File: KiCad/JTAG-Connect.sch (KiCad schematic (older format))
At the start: 2 parts, among them J1 Conn_02x05_Odd_Even, J2 Conn_02x03_Odd_Even

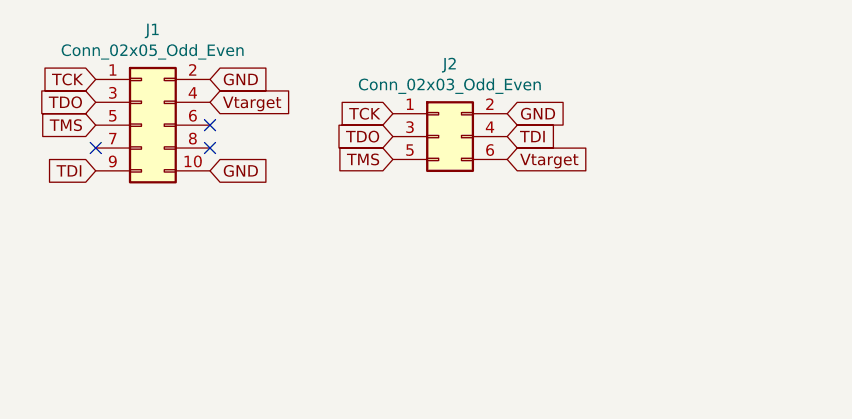
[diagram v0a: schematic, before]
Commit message: updated design
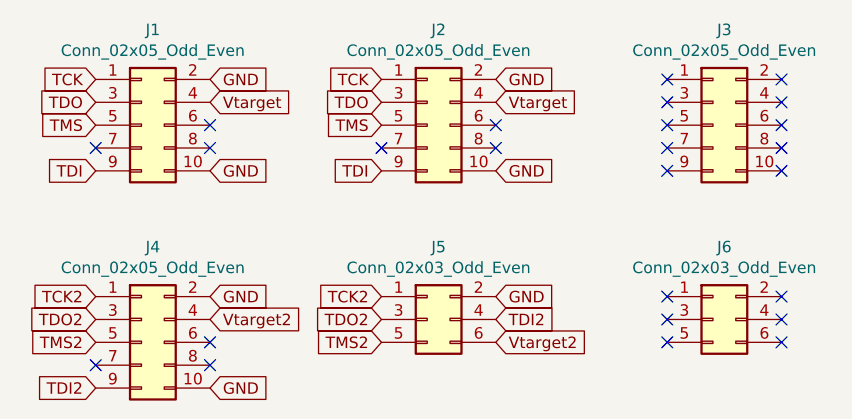
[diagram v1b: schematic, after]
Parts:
- removed J2: Conn_02x03_Odd_Even, Connector_PinHeader_2.00mm:PinHeader_2x03_P2.00mm_Vertical, symbol Connector_Generic:Conn_02x03_Odd_Even
- added J2, J3: Conn_02x05_Odd_Even, JTAG-Connect:PinHeader_2x05_P2.00mm_JTAG_connect_on_SMD_pads, symbol Connector_Generic:Conn_02x05_Odd_Even
- added J4: Conn_02x05_Odd_Even, Connector_IDC:IDC-Header_2x05_P2.54mm_Vertical, symbol Connector_Generic:Conn_02x05_Odd_Even
- added J5, J6: Conn_02x03_Odd_Even, JTAG-Connect:PinHeader_2x03_P2.00mm_JTAG_connect_on_SMD_pads, symbol Connector_Generic:Conn_02x03_Odd_Even
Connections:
- net GND: now also J2.10 (Pin_10), J2.2 (Pin_2), J4.10 (Pin_10), J4.2 (Pin_2), J5.2 (Pin_2)
- net TCK: now also J2.1 (Pin_1)
- net TDI: now also J2.9 (Pin_9)
- net TDO: now also J2.3 (Pin_3)
- net TMS: now also J2.5 (Pin_5)
- net Vtarget: now also J2.4 (Pin_4)
- new net TCK2: J4.1 (Pin_1), J5.1 (Pin_1)
- new net TDI2: J4.9 (Pin_9), J5.4 (Pin_4)
- new net TDO2: J4.3 (Pin_3), J5.3 (Pin_3)
- new net TMS2: J4.5 (Pin_5), J5.5 (Pin_5)
- new net Vtarget2: J4.4 (Pin_4), J5.6 (Pin_6)
- no-connect marks 3 -> 25
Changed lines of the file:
@@
 $EndDescr
-$Comp
-L Connector_Generic:Conn_02x03_Odd_Even J2
-U 1 1 6687D8BE
-P 3650 2650
-F 0 "J2" H 3700 2967 50  0000 C CNN
-F 1 "Conn_02x03_Odd_Even" H 3700 2876 50  0000 C CNN
-F 2 "Connector_PinHeader_2.00mm:PinHeader_2x03_P2.00mm_Vertical" H 3650 2650 50  0001 C CNN
-F 3 "~" H 3650 2650 50  0001 C CNN
-	1    3650 2650
-	1    0    0    -1
-$EndComp
-Text GLabel 3450 2550 0    50   Input ~ 0
-TCK
-Text GLabel 3450 2650 0    50   Input ~ 0
-TDO
-Text GLabel 3450 2750 0    50   Input ~ 0
-TMS
-Text GLabel 3950 2550 2    50   Input ~ 0
-GND
-Text GLabel 3950 2650 2    50   Input ~ 0
-TDI
-Text GLabel 3950 2750 2    50   Input ~ 0
-Vtarget
 $Comp
 L Connector_Generic:Conn_02x05_Odd_Even J1
@@
 TDI
 NoConn ~ 2150 2700
-Text GLabel 2650 2400 2    50   Input ~ 0
+NoConn ~ 2650 2600
+NoConn ~ 2650 2700
+$Comp
+L Connector_Generic:Conn_02x05_Odd_Even J2
+U 1 1 66A23D81
+P 3600 2600
+F 0 "J2" H 3650 3017 50  0000 C CNN
+F 1 "Conn_02x05_Odd_Even" H 3650 2926 50  0000 C CNN
+F 2 "JTAG-Connect:PinHeader_2x05_P2.00mm_JTAG_connect_on_SMD_pads" H 3600 2600 50  0001 C CNN
+F 3 "~" H 3600 2600 50  0001 C CNN
+	1    3600 2600
+	1    0    0    -1
+$EndComp
+Text GLabel 3400 2400 0    50   Input ~ 0
+TCK
+Text GLabel 3400 2500 0    50   Input ~ 0
+TDO
+Text GLabel 3400 2600 0    50   Input ~ 0
+TMS
+Text GLabel 3400 2800 0    50   Input ~ 0
+TDI
+Text GLabel 2650 2800 2    50   Input ~ 0
 GND
 Text GLabel 2650 2500 2    50   Input ~ 0
 Vtarget
-Text GLabel 2650 2800 2    50   Input ~ 0
+Text GLabel 2650 2400 2    50   Input ~ 0
 GND
-NoConn ~ 2650 2600
-NoConn ~ 2650 2700
+Text GLabel 3900 2800 2    50   Input ~ 0
+GND
+Text GLabel 3900 2500 2    50   Input ~ 0
+Vtarget
+Text GLabel 3900 2400 2    50   Input ~ 0
+GND
+NoConn ~ 3400 2700
+NoConn ~ 3900 2600
+NoConn ~ 3900 2700
+$Comp
+L Connector_Generic:Conn_02x05_Odd_Even J3
+U 1 1 66A4E5A1
+P 4850 2600
+F 0 "J3" H 4900 3017 50  0000 C CNN
+F 1 "Conn_02x05_Odd_Even" H 4900 2926 50  0000 C CNN
+F 2 "JTAG-Connect:PinHeader_2x05_P2.00mm_JTAG_connect_on_SMD_pads" H 4850 2600 50  0001 C CNN
+F 3 "~" H 4850 2600 50  0001 C CNN
+	1    4850 2600
+	1    0    0    -1
+$EndComp
+NoConn ~ 4650 2700
+NoConn ~ 5150 2600
+NoConn ~ 5150 2700
+NoConn ~ 4650 2400
+NoConn ~ 4650 2500
+NoConn ~ 4650 2600
+NoConn ~ 4650 2800
+NoConn ~ 5150 2500
+NoConn ~ 5150 2800
+NoConn ~ 5150 2400
+$Comp
+L Connector_Generic:Conn_02x03_Odd_Even J5
+U 1 1 66A79AD5
+P 3600 3450
+F 0 "J5" H 3650 3767 50  0000 C CNN
+F 1 "Conn_02x03_Odd_Even" H 3650 3676 50  0000 C CNN
+F 2 "JTAG-Connect:PinHeader_2x03_P2.00mm_JTAG_connect_on_SMD_pads" H 3600 3450 50  0001 C CNN
+F 3 "~" H 3600 3450 50  0001 C CNN
+	1    3600 3450
+	1    0    0    -1
+$EndComp
+Text GLabel 3400 3350 0    50   Input ~ 0
+TCK2
+Text GLabel 3400 3450 0    50   Input ~ 0
+TDO2
+Text GLabel 3400 3550 0    50   Input ~ 0
+TMS2
+Text GLabel 3900 3350 2    50   Input ~ 0
+GND
+Text GLabel 3900 3450 2    50   Input ~ 0
+TDI2
+NoConn ~ 5150 3550
+NoConn ~ 4650 3350
+NoConn ~ 4650 3450
+NoConn ~ 4650 3550
+NoConn ~ 5150 3450
+NoConn ~ 5150 3350
+Text GLabel 3900 3550 2    50   Input ~ 0
+Vtarget2
+$Comp
+L Connector_Generic:Conn_02x05_Odd_Even J4
+U 1 1 66A89D27
+P 2350 3550
+F 0 "J4" H 2400 3967 50  0000 C CNN
+F 1 "Conn_02x05_Odd_Even" H 2400 3876 50  0000 C CNN
+F 2 "Connector_IDC:IDC-Header_2x05_P2.54mm_Vertical" H 2350 3550 50  0001 C CNN
+F 3 "~" H 2350 3550 50  0001 C CNN
+	1    2350 3550
+	1    0    0    -1
+$EndComp
+Text GLabel 2150 3750 0    50   Input ~ 0
+TDI2
+NoConn ~ 2150 3650
+NoConn ~ 2650 3550
+NoConn ~ 2650 3650
+Text GLabel 2650 3750 2    50   Input ~ 0
+GND
+Text GLabel 2650 3450 2    50   Input ~ 0
+Vtarget2
+Text GLabel 2650 3350 2    50   Input ~ 0
+GND
+Text GLabel 2150 3350 0    50   Input ~ 0
+TCK2
+Text GLabel 2150 3450 0    50   Input ~ 0
+TDO2
+Text GLabel 2150 3550 0    50   Input ~ 0
+TMS2
+$Comp
+L Connector_Generic:Conn_02x03_Odd_Even J6
+U 1 1 66A98FAE
+P 4850 3450
+F 0 "J6" H 4900 3767 50  0000 C CNN
+F 1 "Conn_02x03_Odd_Even" H 4900 3676 50  0000 C CNN
+F 2 "JTAG-Connect:PinHeader_2x03_P2.00mm_JTAG_connect_on_SMD_pads" H 4850 3450 50  0001 C CNN
+F 3 "~" H 4850 3450 50  0001 C CNN
+	1    4850 3450
+	1    0    0    -1
+$EndComp
 $EndSCHEMATC
